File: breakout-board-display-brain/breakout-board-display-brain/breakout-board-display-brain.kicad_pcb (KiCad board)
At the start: 2 copper layers, 55 x 51.5 mm, 5 parts, among them J1 Conn_01x19_Socket, J2 Conn_01x19_Socket, J3 Conn_01x02_Socket, J4 Conn_01x04_Socket, SW1 RotaryEncoder_Switch

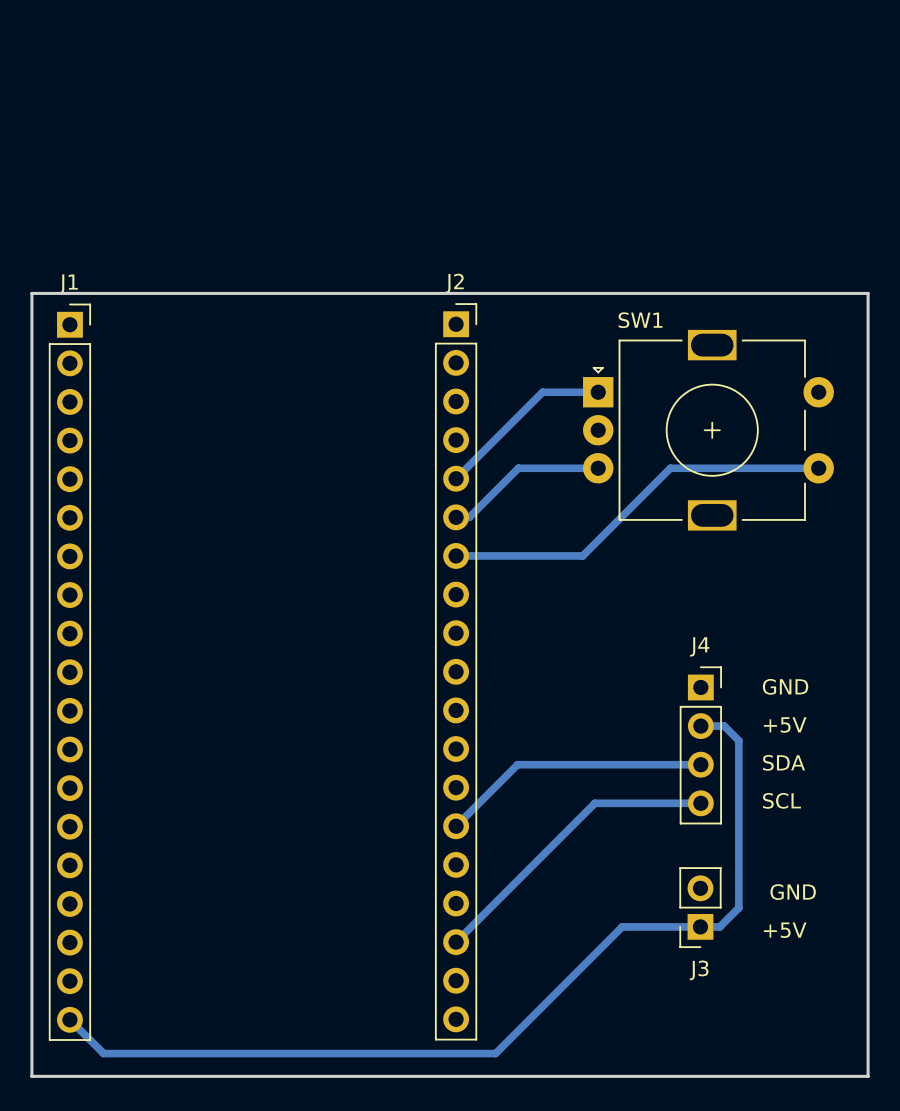
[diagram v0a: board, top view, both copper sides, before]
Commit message: funk breakout board routed
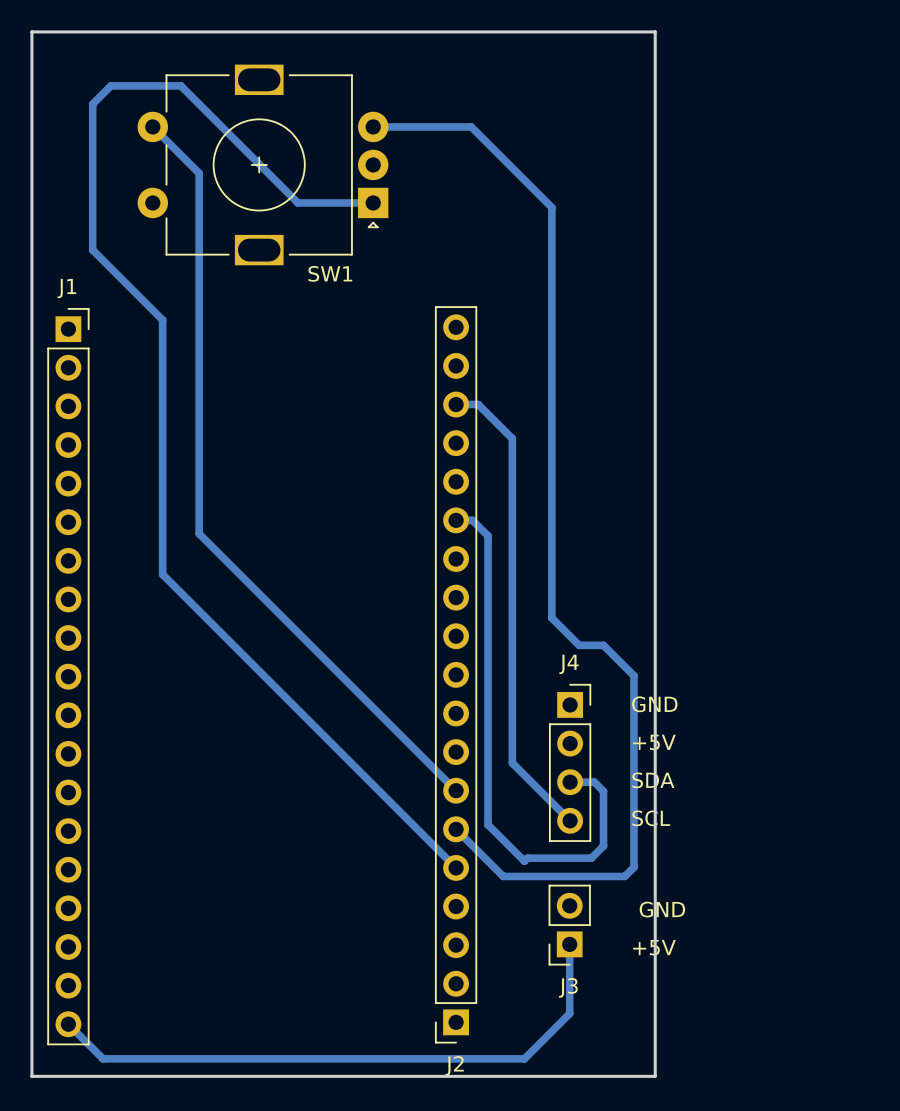
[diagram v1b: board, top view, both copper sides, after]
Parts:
- moved J2 45.9 mm to (154.5, 123.6), turned to 180 degrees
- moved SW1 19.3 mm to (149.1, 69.7), turned to 180 degrees
- moved J3 8.68 mm to (162.0, 118.5)
- moved J4 8.68 mm to (162.0, 102.7)
- moved J1 0.31 mm to (129.0, 78.0)
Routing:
- net /IO2: track 11.7 -> 82.3 mm
- net /IO0: track 10.7 -> 73.8 mm
- net /IO4: track 26.2 -> 51.9 mm
- net +5V: track 62.8 -> 39.7 mm
- net /IO21_SDA: track 17.8 -> 36.6 mm
- net /IO22_SCL: track 19.9 -> 31.3 mm
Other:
- board size 55 x 51.5 mm -> 41 x 68.7 mm

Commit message: Revert "Merge branch 'main' of https://github.com/DominikRzecki/mpm-hardware"
This reverts commit b1fb40005cc6000a652d43f250fbd6541baa0df3, reversing
changes made to 77b873b98367f4cea487d2747d29dc0cf0db4d54.
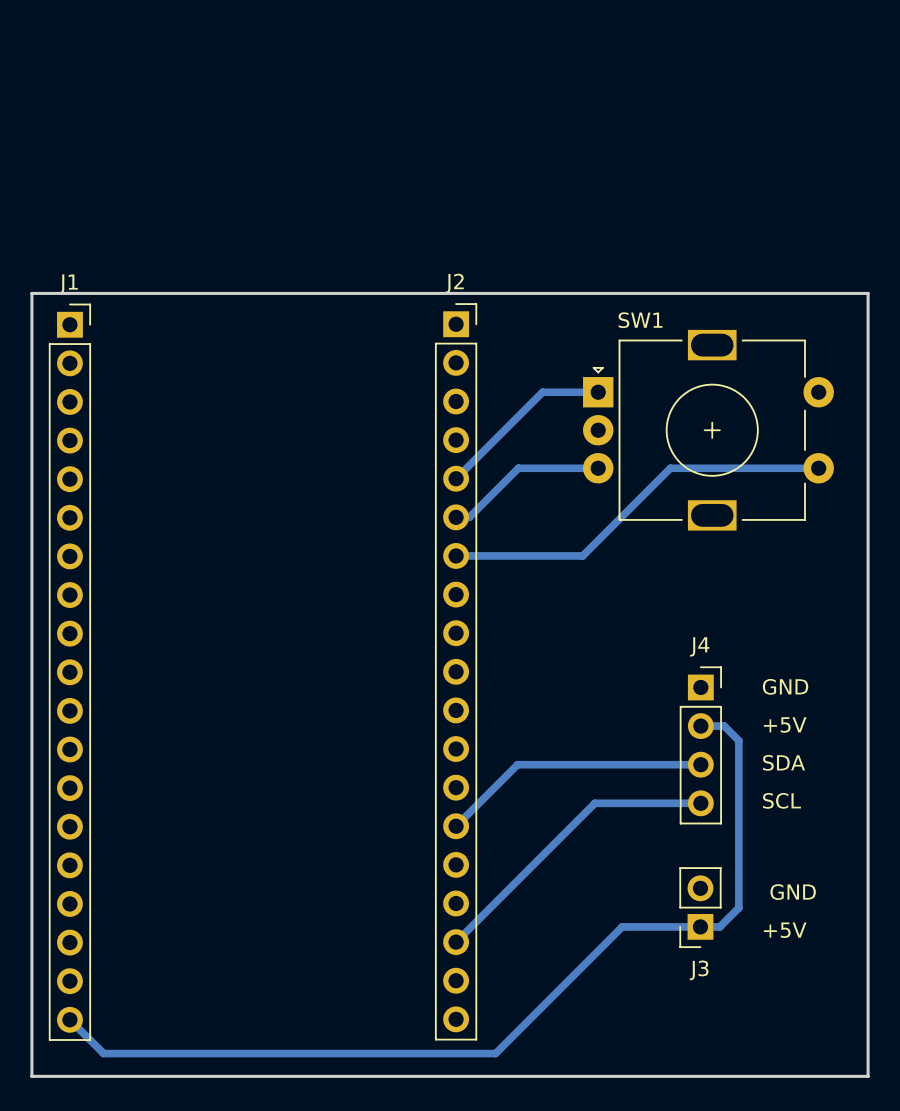
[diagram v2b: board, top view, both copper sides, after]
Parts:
- moved J2 45.9 mm to (154.5, 77.7), turned to 0 degrees
- moved SW1 19.3 mm to (163.8, 82.2), turned to 0 degrees
- moved J3 8.68 mm to (170.6, 117.3)
- moved J4 8.68 mm to (170.6, 101.6)
- moved J1 0.31 mm to (129.1, 77.7)
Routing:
- net /IO2: track 82.3 -> 11.7 mm
- net /IO0: track 73.8 -> 10.7 mm
- net /IO4: track 51.9 -> 26.2 mm
- net +5V: track 39.7 -> 62.8 mm
- net /IO21_SDA: track 36.6 -> 17.8 mm
- net /IO22_SCL: track 31.3 -> 19.9 mm
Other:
- board size 41 x 68.7 mm -> 55 x 51.5 mm
